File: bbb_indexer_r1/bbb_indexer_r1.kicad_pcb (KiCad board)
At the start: 2 copper layers, 54.6 x 86.4 mm, 10 parts, among them J3 SS-60000-008, P8 BeagleBone_Black_Header, P9 BeagleBone_Black_Header

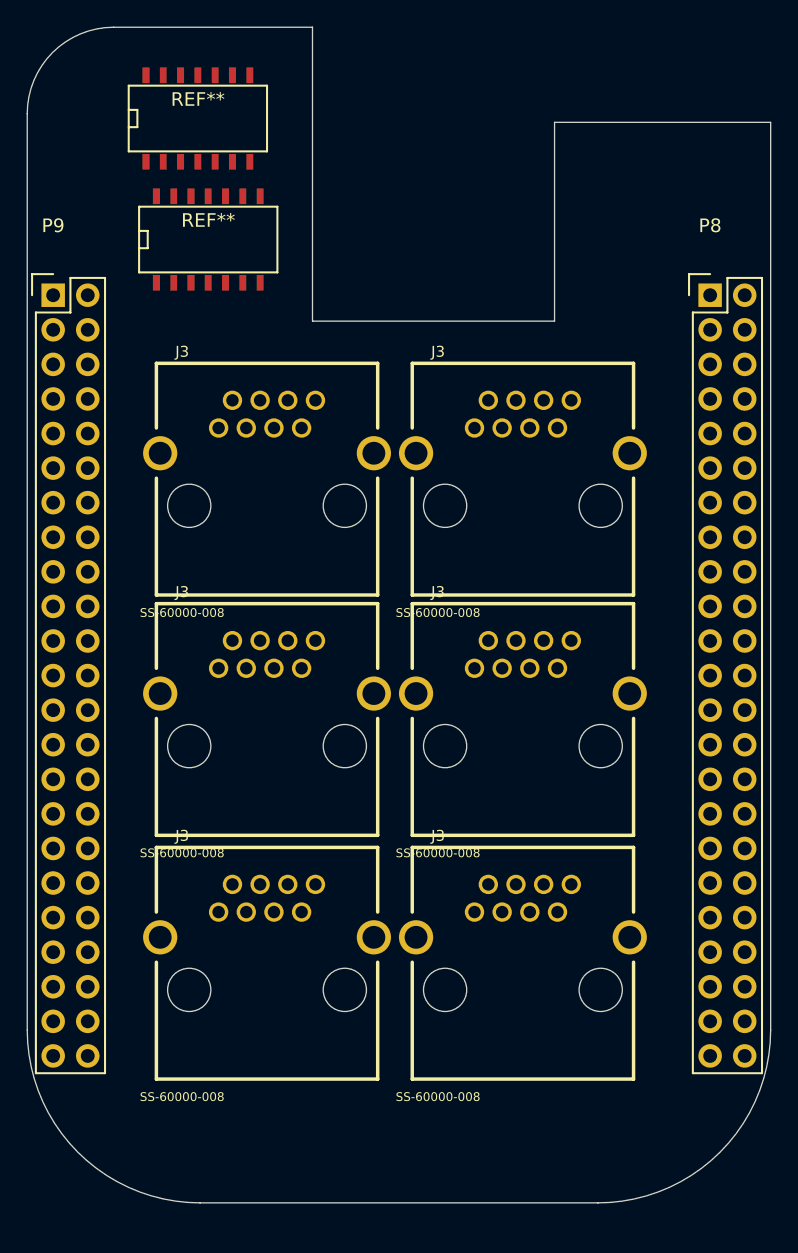
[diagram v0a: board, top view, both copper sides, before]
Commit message: routing mostly complete
Signed-off-by: John McMaster <johndmcmaster@gmail.com>
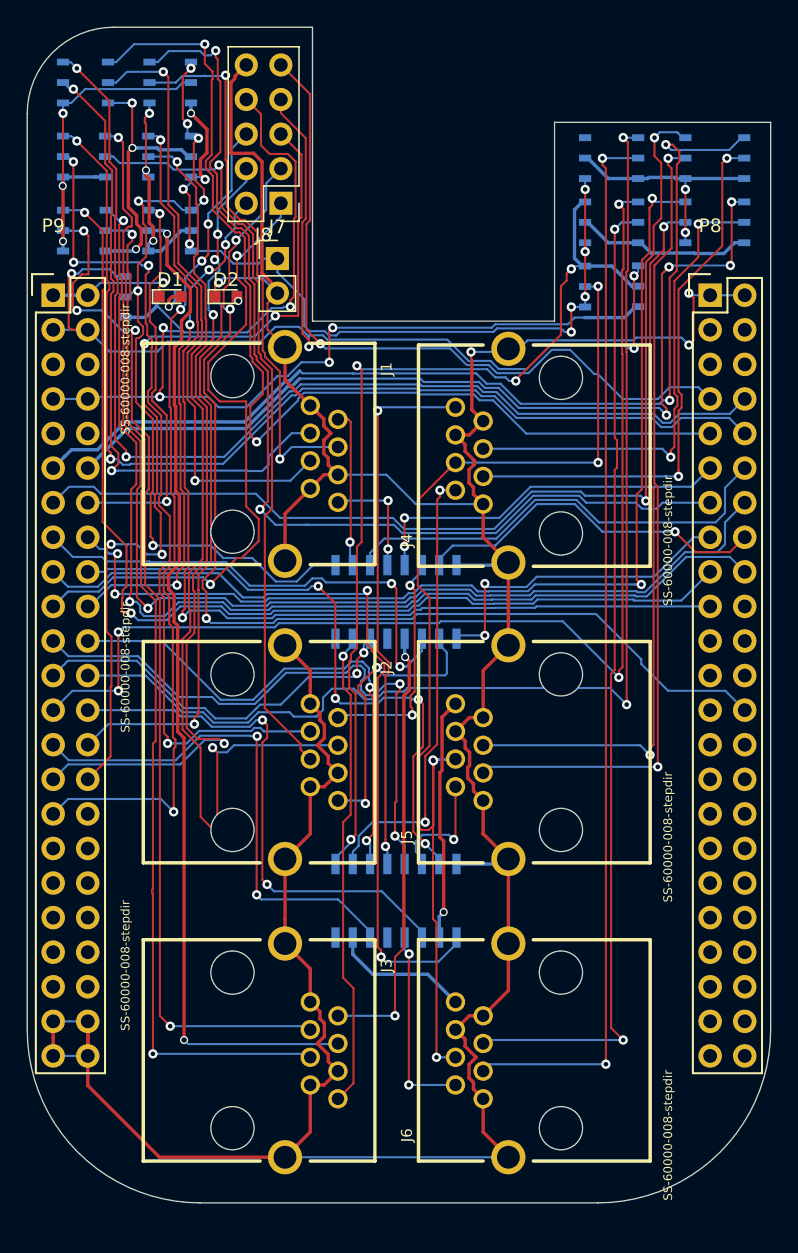
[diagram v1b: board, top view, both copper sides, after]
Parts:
- removed the J3 at (150.9, 95.5)
- removed the J3 at (150.9, 113.4)
- removed the J3 at (150.9, 77.9)
- removed the J3 at (132.1, 113.4)
- removed the J3 at (132.1, 95.5)
- removed the J3 at (132.1, 77.9)
- removed REF** (x2): SOIC-14_N, SMD_Packages:SOIC-14_N
- added D1: LED, LEDs:LED_0603, F.Cu at (125.0, 62.5)
- added D2: LED, LEDs:LED_0603, F.Cu at (129.1, 62.5)
- added J1: SS-60000-008-stepdir, SS-60000-008:520260-4, F.Cu at (129.5, 74.0)
- added J2: SS-60000-008-stepdir, SS-60000-008:520260-4, F.Cu at (129.5, 95.9)
- added J3: SS-60000-008-stepdir, SS-60000-008:520260-4, F.Cu at (129.5, 117.9)
- added J4: SS-60000-008-stepdir, SS-60000-008:520260-4, F.Cu at (153.7, 74.2)
- added J5: SS-60000-008-stepdir, SS-60000-008:520260-4, F.Cu at (153.7, 95.9)
- added J6: SS-60000-008-stepdir, SS-60000-008:520260-4, F.Cu at (153.7, 117.9)
- added J7: Conn_01x02, Pin_Headers:Pin_Header_Straight_1x02_Pitch2.54mm, F.Cu at (132.8, 59.7)
- added J8: Conn_02x05_Odd_Even, Pin_Headers:Pin_Header_Straight_2x05_Pitch2.54mm, F.Cu at (133.1, 55.6)
- added R1: Pad3, lib:R3_0603, B.Cu at (126.5, 46.8)
- added R10: Pad3, lib:R3_0603, B.Cu at (117.1, 57.6)
- added R11: Pad3, lib:R3_0603, B.Cu at (120.2, 57.6)
- added R12: Pad3, lib:R3_0603, B.Cu at (123.4, 57.6)
- added R13: Pad3, lib:R3_0603, B.Cu at (121.7, 62.5)
- added R14: Pad3, lib:R3_0603, B.Cu at (159.3, 61.7)
- added R15: Pad3, lib:R3_0603, B.Cu at (155.4, 52.3)
- added R16: Pad3, lib:R3_0603, B.Cu at (155.4, 57.0)
- added R17: Pad3, lib:R3_0603, B.Cu at (155.4, 61.7)
- added R18: Pad3, lib:R3_0603, B.Cu at (167.1, 52.3)
- added R19: Pad3, lib:R3_0603, B.Cu at (167.1, 57.0)
- added R2: Pad3, lib:R3_0603, B.Cu at (126.5, 52.2)
- added R21: Pad3, lib:R3_0603, B.Cu at (162.8, 52.3)
- added R22: Pad3, lib:R3_0603, B.Cu at (162.8, 57.0)
- added R24: Pad3, lib:R3_0603, B.Cu at (159.3, 52.3)
- added R25: Pad3, lib:R3_0603, B.Cu at (159.3, 57.0)
- added R29: R, Resistors_SMD:R_0603, B.Cu at (124.7, 62.5)
- added R3: Pad3, lib:R3_0603, B.Cu at (126.5, 57.6)
- added R30: R, Resistors_SMD:R_0603, B.Cu at (129.0, 62.5)
- added R4: Pad3, lib:R3_0603, B.Cu at (117.1, 46.8)
- added R5: Pad3, lib:R3_0603, B.Cu at (120.4, 46.8)
- added R6: Pad3, lib:R3_0603, B.Cu at (123.4, 46.8)
- added R7: Pad3, lib:R3_0603, B.Cu at (117.1, 52.2)
- added R8: Pad3, lib:R3_0603, B.Cu at (120.2, 52.2)
- added R9: Pad3, lib:R3_0603, B.Cu at (123.4, 52.2)
- added U1: 4050, Housings_SOIC:SOIC-16_3.9x9.9mm_Pitch1.27mm, B.Cu at (141.6, 84.9)
- added U2: 4050, Housings_SOIC:SOIC-16_3.9x9.9mm_Pitch1.27mm, B.Cu at (141.6, 106.9)
- P8: value BeagleBone_Black_Header -> BeagleBone_Black_Header_P8
- P9: value BeagleBone_Black_Header -> BeagleBone_Black_Header_P9
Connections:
- net GNDA_ADC renamed Net-(P9-Pad34)
- net GNDD renamed GND
- net PWR_BUT renamed Net-(P9-Pad9)
- net SYS_RESETN renamed Net-(P9-Pad10)
- net VDD_ADC renamed Net-(P9-Pad32)
- P8 pad 10: Net-(P8-Pad10) -> /Y-MIN
- P8 pad 11: Net-(P8-Pad11) -> /X-DIR
- P8 pad 12: Net-(P8-Pad12) -> /X-STEP
- P8 pad 13: Net-(P8-Pad13) -> /X-IO
- P8 pad 14: Net-(P8-Pad14) -> /Y-MAX
- P8 pad 15: Net-(P8-Pad15) -> /Y-DIR
- P8 pad 16: Net-(P8-Pad16) -> /Y-STEP
- P8 pad 17: Net-(P8-Pad17) -> /Z-MIN
- P8 pad 18: Net-(P8-Pad18) -> /Z-MAX
- P8 pad 19: Net-(P8-Pad19) -> /Y-IO
- P8 pad 26: Net-(P8-Pad26) -> /LED-STAT
- P8 pad 7: Net-(P8-Pad7) -> /ESTOP
- P8 pad 8: Net-(P8-Pad8) -> /X-MIN
- P8 pad 9: Net-(P8-Pad9) -> /X-MAX
- P9 pad 11: Net-(P9-Pad11) -> /A-MIN
- P9 pad 12: Net-(P9-Pad12) -> /A-MAX
- P9 pad 13: Net-(P9-Pad13) -> /B-MIN
- P9 pad 14: Net-(P9-Pad14) -> /Z-IO
- P9 pad 15: Net-(P9-Pad15) -> /Z-STEP
- P9 pad 16: Net-(P9-Pad16) -> /B-MAX
- P9 pad 17: Net-(P9-Pad17) -> /B-DIR
- P9 pad 18: Net-(P9-Pad18) -> /B-STEP
- P9 pad 19: Net-(P9-Pad19) -> /GPIO1
- P9 pad 20: Net-(P9-Pad20) -> /GPIO2
- P9 pad 21: Net-(P9-Pad21) -> /A-DIR
- P9 pad 22: Net-(P9-Pad22) -> /A-STEP
- P9 pad 23: Net-(P9-Pad23) -> /Z-DIR
- P9 pad 24: Net-(P9-Pad24) -> /C-MIN
- P9 pad 25: Net-(P9-Pad25) -> /C-MAX
- P9 pad 26: Net-(P9-Pad26) -> /C-STEP
- P9 pad 27: Net-(P9-Pad27) -> /C-DIR
- P9 pad 28: Net-(P9-Pad28) -> /GPIO3
- P9 pad 29: Net-(P9-Pad29) -> /GPIO4
- P9 pad 30: Net-(P9-Pad30) -> /GPIO5
- P9 pad 31: Net-(P9-Pad31) -> /GPIO6
- P9 pad 5: +5V -> Net-(P9-Pad5)
- P9 pad 6: +5V -> Net-(P9-Pad6)
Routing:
- net GND: track 0.00 -> 270.8 mm, vias 0 -> 5
- net SYS_5V: track 0.00 -> 87.2 mm, vias 0 -> 5
- net /C-MIN: track 0.00 -> 87.0 mm, vias 0 -> 2
- net /Y-MAX: track 0.00 -> 86.4 mm, vias 0 -> 2
- net /R-V3: track 0.00 -> 86.0 mm, vias 0 -> 5
- net /C-MAX: track 0.00 -> 85.0 mm, vias 0 -> 4
- net +3V3: track 0.00 -> 82.4 mm, vias 0 -> 4
- net /X-MIN: track 0.00 -> 81.0 mm, vias 0 -> 2
- net /Z-MAX: track 0.00 -> 79.7 mm, vias 0 -> 2
- net Net-(J6-Pad3): track 0.00 -> 78.5 mm, vias 0 -> 2
- net /Z-MIN: track 0.00 -> 78.3 mm, vias 0 -> 2
- net /Y-IO: track 0.00 -> 77.6 mm, vias 0 -> 2
- net /X-IO: track 0.00 -> 77.6 mm, vias 0 -> 2
- net /B-MAX: track 0.00 -> 77.0 mm, vias 0 -> 4
- net /Y-MIN: track 0.00 -> 76.7 mm, vias 0 -> 2
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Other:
- net class Default: clearance 0.2 -> 0.1524; trace_width 0.25 -> 0.1524; via_dia 0.6 -> 0.6858; via_drill 0.4 -> 0.3302
- rule trace_clearance: 0.2 -> 0.1524
- rule trace_min: 0.2 -> 0.1524
- rule via_min_drill: 0.3 -> 0.254
- rule via_min_size: 0.4 -> 0.508
